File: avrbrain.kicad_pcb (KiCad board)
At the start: 2 copper layers, 85 x 56 mm, 46 parts, among them J1 XKTF-0803-0, J12 PD/PE, J2 U254-051T-4BH81-S2S, J4 UPDI, J5 UEXT, J6 PC, J7 PA/PB, J8 PG, J9 SM04B-SRSS-TB, Q1 BSS138, SW1 RESET, SW2 VDD, U1 CH340C, U2 AVR128DB64x-xPT, U3 PCF8563T, U5 AMS1117-3.3, Y1 32kHz

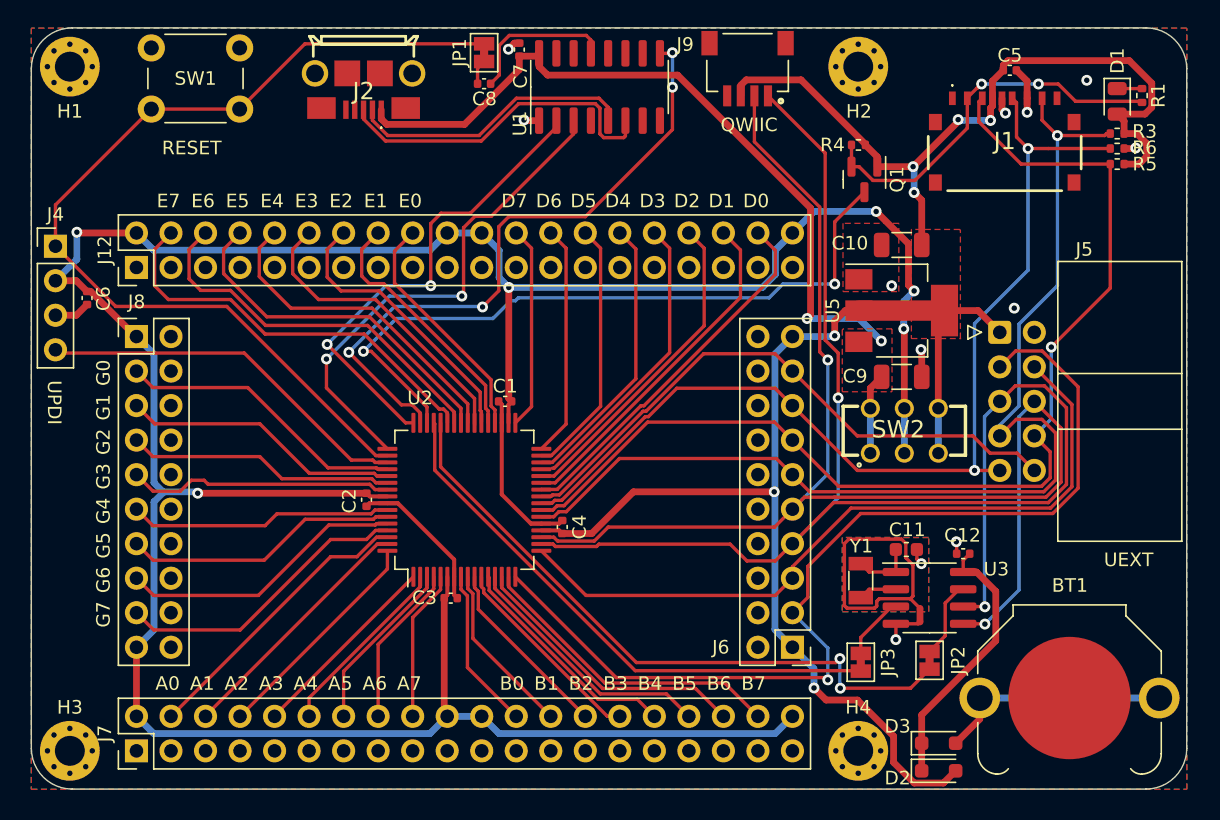
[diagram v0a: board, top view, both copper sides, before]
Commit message: Finish layout and routing
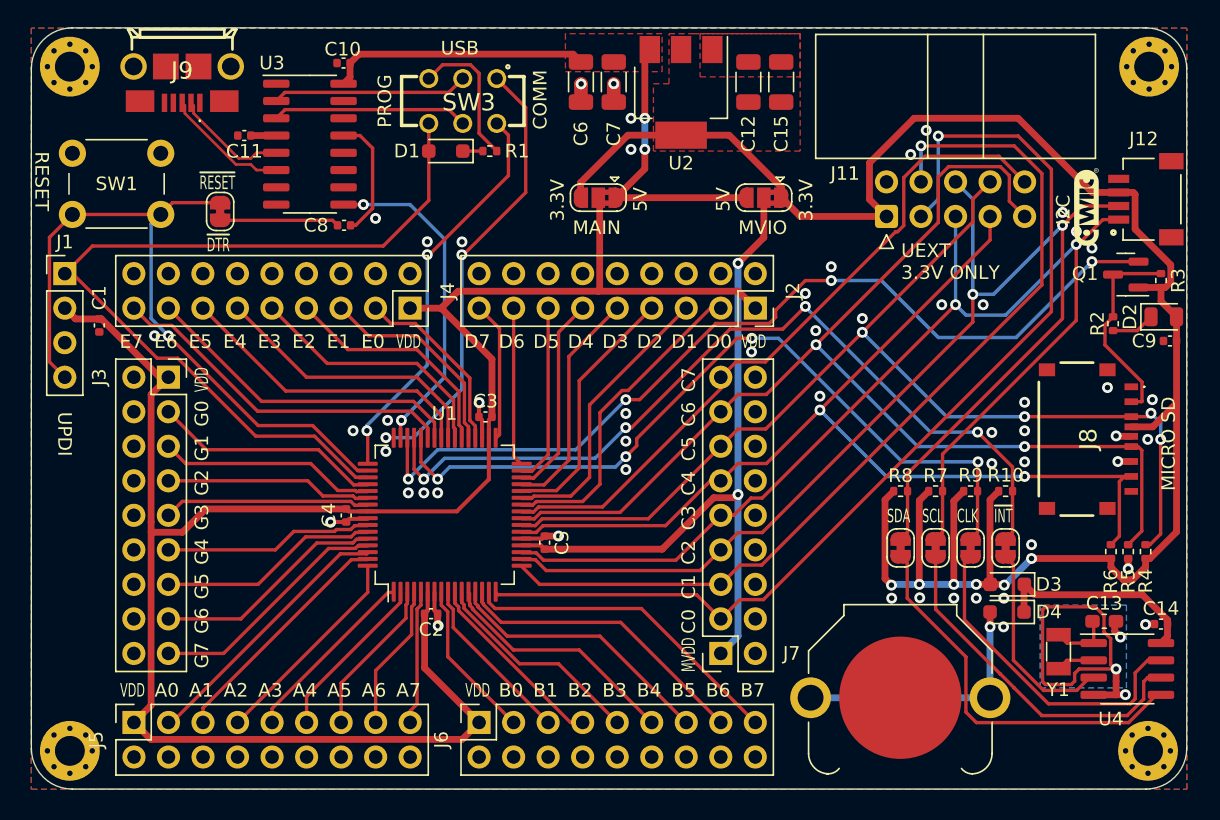
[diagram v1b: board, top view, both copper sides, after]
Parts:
- removed SW2: VDD, SamacSys_Parts:JS202011CQN
- removed U5: AMS1117-3.3, Package_TO_SOT_SMD:SOT-223-3_TabPin2
- added C13: 27pf, Capacitor_SMD:C_0603_1608Metric_Pad1.08x0.95mm_HandSolder, F.Cu at (200.9, 124.6)
- added C14: 0.1uf, Capacitor_SMD:C_0402_1005Metric, F.Cu at (205.1, 124.8)
- added C15: 22uf, Capacitor_SMD:C_1206_3216Metric, F.Cu at (177.2, 85.0)
- added D4: 1N5819WS, Diode_SMD:D_SOD-323_HandSoldering, F.Cu at (193.8, 124.0)
- added J11: UEXT, Connector_IDC:IDC-Header_2x05_P2.54mm_Horizontal, F.Cu at (184.9, 94.9)
- added J3: PORTG, Connector_PinSocket_2.54mm:PinSocket_2x09_P2.54mm_Vertical, F.Cu at (132.1, 106.7)
- added JP4: VDD_MAIN, Jumper:SolderJumper-3_P1.3mm_Bridged2Bar12_RoundedPad1.0x1.5mm, F.Cu at (163.7, 93.5)
- added JP5: VDD_MVIO, Jumper:SolderJumper-3_P1.3mm_Bridged2Bar12_RoundedPad1.0x1.5mm, F.Cu at (175.9, 93.5)
- added JP6: RTC_CLK, Jumper:SolderJumper-2_P1.3mm_Bridged_RoundedPad1.0x1.5mm, F.Cu at (191.1, 119.2)
- added JP7: RTC_INT, Jumper:SolderJumper-2_P1.3mm_Bridged_RoundedPad1.0x1.5mm, F.Cu at (193.7, 119.2)
- added R10: 2.2K, Resistor_SMD:R_0402_1005Metric, F.Cu at (193.7, 115.1)
- added R2: 1K, Resistor_SMD:R_0402_1005Metric, F.Cu at (201.6, 102.7)
- added R7: 2.2K, Resistor_SMD:R_0402_1005Metric, F.Cu at (188.5, 115.1)
- added R8: 2.2K, Resistor_SMD:R_0402_1005Metric, F.Cu at (186.0, 115.1)
- added R9: 2.2K, Resistor_SMD:R_0402_1005Metric, F.Cu at (191.1, 115.1)
- added SW3: PROG_EN, SamacSys_Parts:JS202011CQN, F.Cu at (153.7, 86.4)
- added U4: PCF8563T, Package_SO:SOIC-8_3.9x4.9mm_P1.27mm, F.Cu at (202.6, 128.1)
- C10, C9: value 1uf -> 0.1uf; footprint Capacitor_SMD:C_1206_3216Metric -> Capacitor_SMD:C_0402_1005Metric
- C11: value 27pf -> 0.1uf; footprint Capacitor_SMD:C_0603_1608Metric -> Capacitor_SMD:C_0402_1005Metric
- C12, C7: value 0.1uf -> 1uf; footprint Capacitor_SMD:C_0402_1005Metric -> Capacitor_SMD:C_1206_3216Metric
- C6: value 0.1uf -> 22uf; footprint Capacitor_SMD:C_0402_1005Metric -> Capacitor_SMD:C_1206_3216Metric
- D1: value LED -> 1N5819WS; footprint LED_SMD:LED_0805_2012Metric -> Diode_SMD:D_SOD-323_HandSoldering
- D2: value 1N5819WS -> LED; footprint Diode_SMD:D_SOD-323_HandSoldering -> LED_SMD:LED_0805_2012Metric
- J1: value XKTF-0803-0 -> UPDI; footprint SamacSys_Parts:XKTF08030 -> Connector_PinHeader_2.54mm:PinHeader_1x04_P2.54mm_Vertical
- J12: value PD/PE -> SM04B-SRSS-TB; footprint Connector_PinHeader_2.54mm:PinHeader_2x20_P2.54mm_Vertical -> Custom:JST_SM04B-SRSS-TB_LF__SN_
- J2: value U254-051T-4BH81-S2S -> PORTD; footprint SamacSys_Parts:U254051T4BH81S2S -> Connector_PinSocket_2.54mm:PinSocket_2x09_P2.54mm_Vertical
- J4: value UPDI -> PORTE; footprint Connector_PinHeader_2.54mm:PinHeader_1x04_P2.54mm_Vertical -> Connector_PinSocket_2.54mm:PinSocket_2x09_P2.54mm_Vertical
- J5: value UEXT -> PORTA; footprint Connector_IDC:IDC-Header_2x05_P2.54mm_Horizontal -> Connector_PinSocket_2.54mm:PinSocket_2x09_P2.54mm_Vertical
- J6: value PC -> PORTB; footprint Connector_PinHeader_2.54mm:PinHeader_2x10_P2.54mm_Vertical -> Connector_PinSocket_2.54mm:PinSocket_2x09_P2.54mm_Vertical
- J7: value PA/PB -> PORTC; footprint Connector_PinHeader_2.54mm:PinHeader_2x20_P2.54mm_Vertical -> Connector_PinSocket_2.54mm:PinSocket_2x09_P2.54mm_Vertical
- J8: value PG -> XKTF-0803-0; footprint Connector_PinHeader_2.54mm:PinHeader_2x10_P2.54mm_Vertical -> SamacSys_Parts:XKTF08030
- J9: value SM04B-SRSS-TB -> U254-051T-4BH81-S2S; footprint Custom:JST_SM04B-SRSS-TB_LF__SN_ -> SamacSys_Parts:U254051T4BH81S2S
- JP1: footprint Jumper:SolderJumper-2_P1.3mm_Bridged_Pad1.0x1.5mm -> Jumper:SolderJumper-2_P1.3mm_Bridged_RoundedPad1.0x1.5mm
- JP2: value CLK32K -> RTC_SCL; footprint Jumper:SolderJumper-2_P1.3mm_Bridged_Pad1.0x1.5mm -> Jumper:SolderJumper-2_P1.3mm_Bridged_RoundedPad1.0x1.5mm
- JP3: value RTCINT -> RTC_SDA; footprint Jumper:SolderJumper-2_P1.3mm_Bridged_Pad1.0x1.5mm -> Jumper:SolderJumper-2_P1.3mm_Bridged_RoundedPad1.0x1.5mm
- R1: value 1K -> 4.7K
- U1: value CH340C -> AVR128DB64x-xPT; footprint Package_SO:SOIC-16_3.9x9.9mm_P1.27mm -> Package_QFP:TQFP-64_10x10mm_P0.5mm
- U2: value AVR128DB64x-xPT -> AMS1117-3.3; footprint Package_QFP:TQFP-64_10x10mm_P0.5mm -> Package_TO_SOT_SMD:SOT-223-3_TabPin2
- U3: value PCF8563T -> CH340C; footprint Package_SO:SOIC-8_3.9x4.9mm_P1.27mm -> Package_SO:SOIC-16_3.9x9.9mm_P1.27mm
- moved J12 72.4 mm to (202.0, 93.6)
- moved J8 70.2 mm to (199.5, 111.2), turned to 90 degrees
- moved J5 69.9 mm to (129.6, 132.1), turned to 90 degrees
- moved J1 69.8 mm to (124.5, 99.1), turned to 0 degrees
- moved C11 57.4 mm to (137.7, 88.9)
- moved U3 56.5 mm to (142.5, 89.5)
- moved D1 49.5 mm to (152.5, 90.0), turned to 180 degrees
- moved C5 48.8 mm to (159.8, 118.8), turned to 90 degrees
- moved R1 48.2 mm to (155.7, 90.0), turned to 180 degrees
- moved J7 43.6 mm to (172.7, 127.0), turned to 180 degrees
- moved C10 43.2 mm to (145.0, 83.6)
- moved J9 41.6 mm to (133.1, 84.1)
- moved C6 39.7 mm to (162.4, 85.0)
- moved C12 38.1 mm to (174.8, 85.0), turned to 90 degrees
- moved D2 37.3 mm to (205.3, 102.2)
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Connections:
- C10 pad 1: +3.3V -> +5V
- C11 pad 1: GND1 -> Net-(U3-V3)
- C11 pad 2: Net-(U3-OSCI) -> GND
- C12 pad 1: Net-(D2-K) -> +3.3V
- C4 pad 1: +3.3V -> VDD
- C5 pad 1: +3.3V -> VDDF
- C6 pad 1: VDD -> +5V
- C8 pad 1: /~{DTR} -> Net-(U3-~{DTR})
- C9 pad 1: +5V -> +3.3V
- D1 pad 2: +3.3V -> UPDI
- D3 pad 1: Net-(D2-K) -> Net-(D3-K)
- D3 pad 2: Net-(BT1-+) -> +3.3V
- J12 pad 1: GND -> SCL
- J12 pad 2: VDD -> SDA
- J12 pad 3: GND -> +3.3V
- J12 pad 4: /PE7 -> GND
- J2 pad 1: +5V -> VDD
- J2 pad 2: Net-(J2-D-) -> GND
- J2 pad 3: Net-(J2-D+) -> /PD0
- J2 pad 4: unconnected-(J2-ID-Pad4) -> GND
- J2 pad 5: GND -> /PD1
- J4 pad 1: Net-(J4-Pin_1) -> VDD
- J4 pad 2: VDD -> GND
- J4 pad 3: GND -> /PE0
- J4 pad 4: Net-(J4-Pin_4) -> GND
- J5 pad 1: +3.3V -> VDD
- J5 pad 10: /~{UXCS} -> GND
- J5 pad 3: /TX3V -> /PA0
- J5 pad 4: /RX3V -> GND
- J5 pad 5: /SCL -> /PA1
- J5 pad 6: /SDA -> GND
- J5 pad 7: /MISO -> /PA2
- J5 pad 8: /MOSI -> GND
- J5 pad 9: /SCK -> /PA3
- J6 pad 1: +3.3V -> VDD
- J6 pad 11: /MISO -> /PB4
- J6 pad 13: /MOSI -> /PB5
- J6 pad 15: /SCK -> /PB6
- J6 pad 17: /~{UXCS} -> /PB7
- J6 pad 3: /TX3V -> /PB0
- J6 pad 5: /RX3V -> /PB1
- J6 pad 7: /SCL -> /PB2
- J6 pad 9: /SDA -> /PB3
- J7 pad 1: GND -> VDDF
- J7 pad 10: /PA3 -> GND
- J7 pad 11: GND -> MISO
- J7 pad 12: /PA4 -> GND
- J7 pad 13: GND -> MOSI
- J7 pad 14: /PA5 -> GND
- J7 pad 15: GND -> SCK
- J7 pad 16: /PA6 -> GND
- J7 pad 17: GND -> ~{CS}
- J7 pad 18: /PA7 -> GND
- J7 pad 2: VDD -> GND
- J7 pad 3: GND -> TXC
- J7 pad 4: /PA0 -> GND
- J7 pad 5: GND -> RXC
- J7 pad 6: /PA1 -> GND
- J7 pad 7: GND -> SDA
- J7 pad 8: /PA2 -> GND
- J7 pad 9: GND -> SCL
- J9 pad 1: /SCL -> unconnected-(J9-VBUS-Pad1)
- J9 pad 2: /SDA -> /Peripherals/UD-
- J9 pad 3: +3.3V -> /Peripherals/UD+
- J9 pad 4: GND -> unconnected-(J9-ID-Pad4)
- JP1 pad 2: Net-(J4-Pin_1) -> ~{RESET}
- JP2 pad 1: /CLK32K -> SCL
- JP3 pad 1: /~{RTCINT} -> SDA
- Q1 pad 2: Net-(J1-DAT3/CD) -> ~{SDCS}
- Q1 pad 3: /~{SDCS} -> Net-(J8-DAT3/CD)
- R1 pad 1: Net-(J1-DAT3/CD) -> Net-(SW3A-C)
- R3 pad 2: /MISO -> Net-(J8-DAT3/CD)
- R4 pad 2: Net-(J1-DAT3/CD) -> MOSI
- R5 pad 1: +3.3V -> GND
- R5 pad 2: /MOSI -> SCK
- R6 pad 1: GND -> +3.3V
- R6 pad 2: /SCK -> MISO
- SW1 pad 2: Net-(J4-Pin_1) -> ~{RESET}
- U1 pad 1: GND -> /PA3
- U1 pad 10: unconnected-(U1-~{DSR}-Pad10) -> /PB2
- U1 pad 11: unconnected-(U1-~{RI}-Pad11) -> /PB3
- U1 pad 12: unconnected-(U1-~{DCD}-Pad12) -> /PB4
- U1 pad 13: /~{DTR} -> /PB5
- U1 pad 14: /~{RTS} -> /PB6
- U1 pad 15: unconnected-(U1-R232-Pad15) -> /PB7
- U1 pad 16: +5V -> TXC
- U1 pad 2: /RXU -> /PA4
- U1 pad 3: /TXU -> /PA5
- U1 pad 4: unconnected-(U1-V3-Pad4) -> /PA6
- U1 pad 5: Net-(J2-D-) -> /PA7
- U1 pad 6: Net-(J2-D+) -> VDD
- U1 pad 7: unconnected-(U1-NC-Pad7) -> GND
- U1 pad 8: unconnected-(U1-NC-Pad8) -> /PB0
- U1 pad 9: /~{CTS} -> /PB1
- U2 pad 1: /PA3 -> GND
- U2 pad 2: /PA4 -> +3.3V
- U2 pad 3: /PA5 -> +5V
- U3 pad 1: Net-(U3-OSCI) -> GND
- U3 pad 2: Net-(U3-OSCO) -> /Peripherals/USBTX
- U3 pad 3: Net-(JP3-B) -> /Peripherals/USBRX
- U3 pad 4: GND -> Net-(U3-V3)
- U3 pad 5: /SDA -> /Peripherals/UD-
- U3 pad 6: /SCL -> /Peripherals/UD+
- U3 pad 7: Net-(JP2-B) -> unconnected-(U3-NC-Pad7)
- U3 pad 8: Net-(D2-K) -> unconnected-(U3-NC-Pad8)
- Y1 pad 1: Net-(U3-OSCO) -> Net-(U4-OSCO)
- Y1 pad 2: Net-(U3-OSCI) -> Net-(U4-OSCI)
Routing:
- net /SCL: track 107.0 -> 0.00 mm, vias 2 -> 0
- net /SDA: track 100.1 -> 0.00 mm, vias 2 -> 0
- net SDA: track 0.00 -> 93.4 mm, vias 0 -> 2
- net SCL: track 0.00 -> 87.6 mm, vias 0 -> 2
- net SCK: track 0.00 -> 86.8 mm, vias 0 -> 2
- net /MOSI: track 81.0 -> 0.00 mm, vias 1 -> 0
- net /MISO: track 80.5 -> 0.00 mm, vias 1 -> 0
- net MOSI: track 0.00 -> 80.4 mm, vias 0 -> 4
- net TXC: track 0.00 -> 77.3 mm, vias 0 -> 1
- net MISO: track 0.00 -> 76.0 mm, vias 0 -> 2
- net /SCK: track 75.3 -> 0.00 mm, vias 2 -> 0
- net /TX3V: track 73.1 -> 0.00 mm, vias 1 -> 0
- net Net-(J4-Pin_1): track 70.3 -> 0.00 mm
- net RXC: track 0.00 -> 68.5 mm, vias 0 -> 1
- net ~{SDCS}: track 0.00 -> 67.2 mm, vias 0 -> 4
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- removed copper zone on F.Cu, net GND1
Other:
- board text added: "1117-3.3"
- board text added: "3.3V"
- board text added: "5V"
- board text added: "C0"
- board text added: "C1"
- board text added: "C2"
- board text added: "C3"
- board text added: "C4"
- board text added: "C5"
- board text added: "C6"
- board text added: "C7"
- board text added: "CH340C"
- board text added: "CLK"
- board text added: "COMM"
- board text added: "CR1216"
- board text added: "Copyright (C)2024 J.B. Langston III https://github.com/jblang/avrbrain"
- board text added: "I2C"
- board text added: "MAIN"
- board text added: "MICRO SD"
- board text added: "MVDD"
- board text added: "MVIO"
- board text added: "PCF8563"
- board text added: "PROG"
- board text added: "SCL"
- board text added: "SDA"
- board text added: "UEXT 3.3V ONLY"
- board text added: "USB"
- board text added: "VDD"
- board text added: "~{DTR}"
- board text added: "~{INT}"
- board text added: "~{RESET}"
- board text removed: "AVRbrain Copyright (C)2024 J.B. Langston III https://github.com/jblang/avrbrain"
- board text removed: "QWIIC"
- board text removed: "UEXT"
